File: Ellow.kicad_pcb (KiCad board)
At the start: 2 copper layers, 24.3 x 40.6 mm, 23 parts, among them J1 USB_C_Receptacle_USB2.0, J2 M_2_AKey_KB, Q1 A03407, Q2 A03407, U1 AP2112K-3.3, U2 E73-2G4M08S1C, U3 LN2054Y42AMR, Y1 32.768kHz

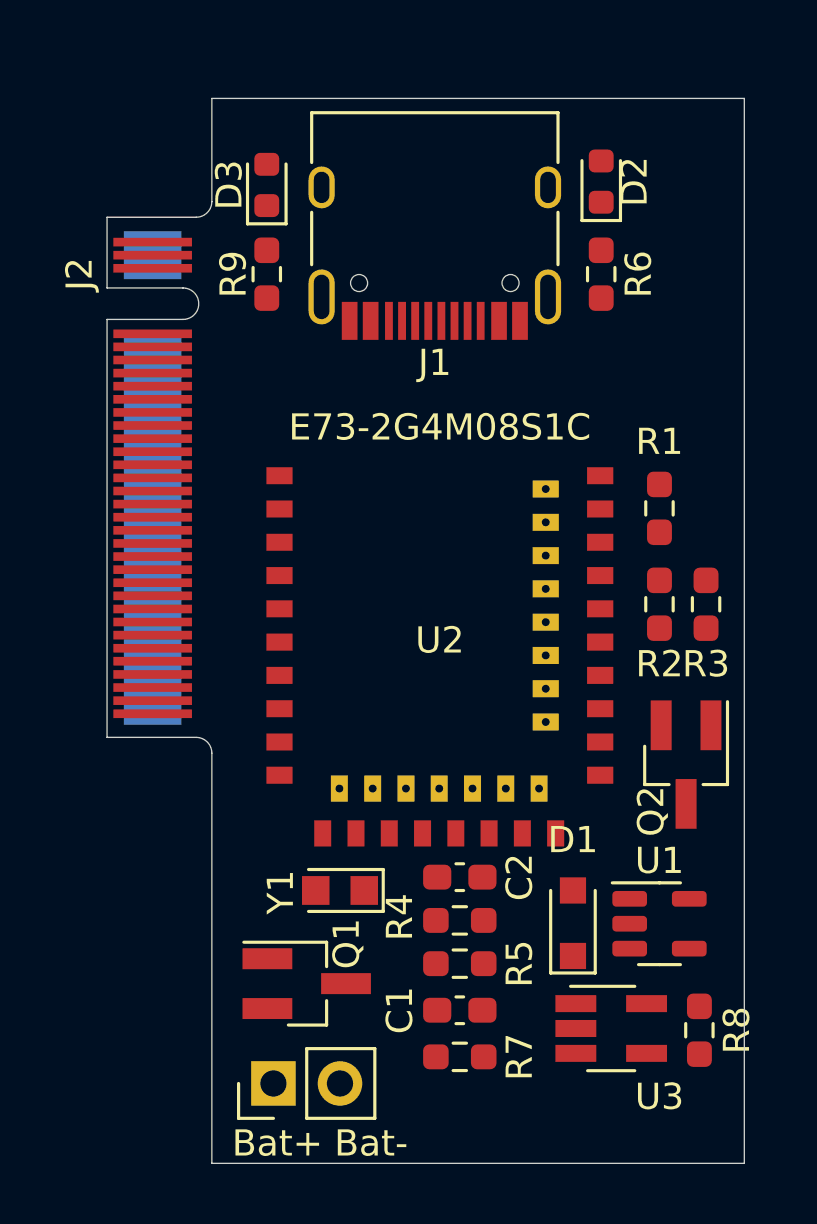
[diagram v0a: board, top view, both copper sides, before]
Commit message: starting to look at routing
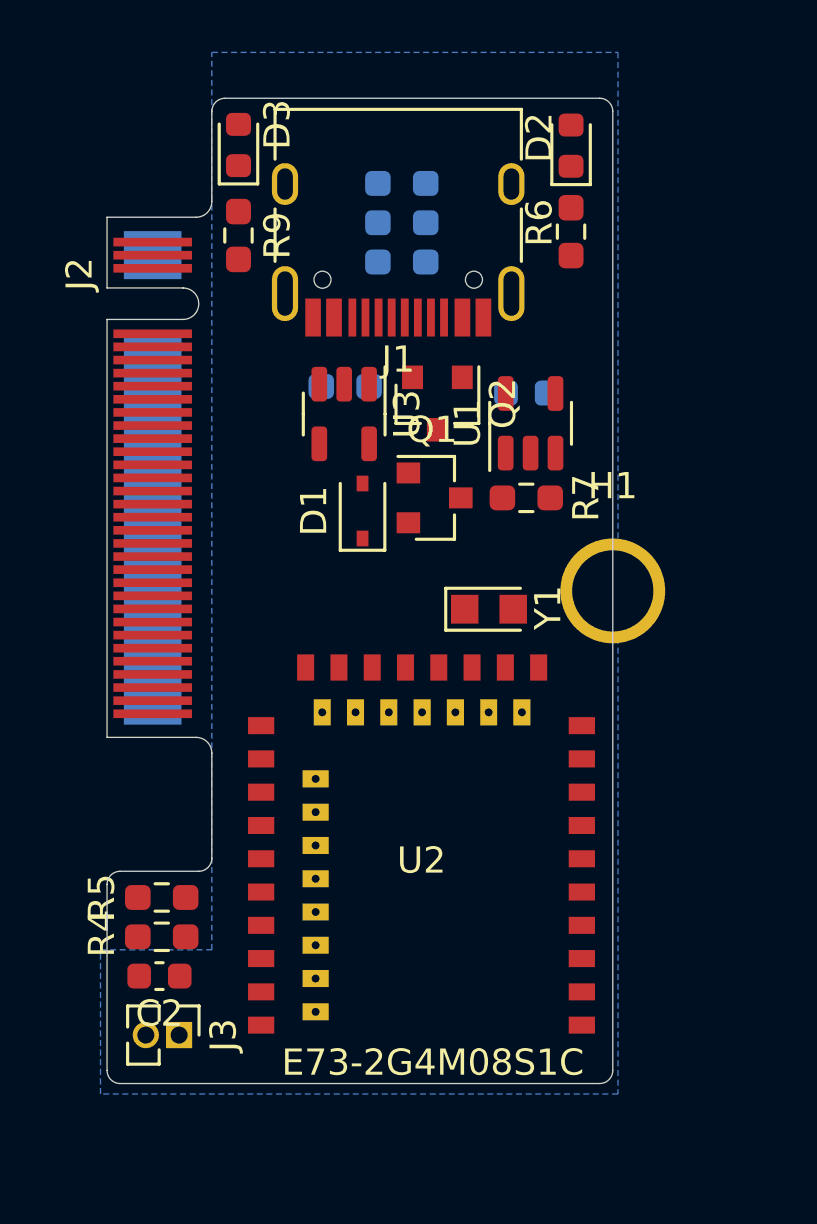
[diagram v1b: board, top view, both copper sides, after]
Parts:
- added H1: MountingHole, ellow:MountingHole_M.2_3mm, F.Cu at (244.1, 107.2)
- C1: footprint Capacitor_SMD:C_0603_1608Metric_Pad1.08x0.95mm_HandSolder -> Capacitor_SMD:C_0603_1608Metric; moved to B.Cu
- C2: footprint Capacitor_SMD:C_0603_1608Metric_Pad1.08x0.95mm_HandSolder -> Capacitor_SMD:C_0603_1608Metric
- D1: footprint Diode_SMD:D_SOD-323_HandSoldering -> Diode_SMD:D_SOD-323
- J3: renamed from Bat+ Bat-; footprint Connector_PinHeader_2.54mm:PinHeader_1x02_P2.54mm_Vertical -> Connector_PinHeader_1.27mm:PinHeader_1x02_P1.27mm_Vertical
- Q1, Q2: footprint Package_TO_SOT_SMD:SOT-23_Handsoldering -> Package_TO_SOT_SMD:SOT-23
- R1, R2, R3, R8: moved to B.Cu
- U3: footprint Package_TO_SOT_SMD:SOT-23-5_HandSoldering -> Package_TO_SOT_SMD:SOT-23-5
- moved R8 28.0 mm to (233.9, 99.4), turned to 180 degrees
- moved U3 25.6 mm to (233.8, 100.5), turned to 270 degrees
- moved C1 23.7 mm to (240.8, 99.7)
- moved R7 21.5 mm to (240.8, 103.7)
- moved R3 19.8 mm to (236.0, 91.7), turned to 0 degrees
- moved U1 19.7 mm to (241.0, 100.8), turned to 90 degrees
- moved Q1 19.2 mm to (237.3, 103.7)
- moved D1 17.7 mm to (234.5, 104.2)
- moved Q2 16.7 mm to (237.4, 100.1)
- moved R2 16.3 mm to (236.0, 94.7), turned to 180 degrees
- moved R1 14.7 mm to (236.0, 93.2), turned to 0 degrees
- moved Y1 12.1 mm to (239.4, 107.9), turned to 0 degrees
- moved C2 12.1 mm to (226.8, 121.9)
- moved R5 11.7 mm to (226.9, 118.9), turned to 180 degrees
- moved R4 11.4 mm to (226.9, 120.4)
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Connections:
- net Net-(U2-Pad12) renamed P0.26
- net Net-(U2-Pad14) renamed P0.06
- net Net-(U2-Pad20) renamed P0.12
- net Net-(U2-Pad22) renamed 90.07
- net Net-(U2-Pad34) renamed P0.22
- net Net-(U2-Pad36) renamed P1.00
- net Net-(U2-Pad38) renamed P1.02
- net Net-(U2-Pad40) renamed P1.04
- J2 pad 1: (no net) -> GND
- J2 pad 16: (no net) -> P0.31
- J2 pad 17: (no net) -> P0.30
- J2 pad 18: (no net) -> Net-(J2-Pad18)
- J2 pad 19: (no net) -> Net-(J2-Pad19)
- J2 pad 2: (no net) -> EXT_VCC
- J2 pad 20: (no net) -> P0.29
- J2 pad 21: (no net) -> P0.02
- J2 pad 22: (no net) -> Net-(J2-Pad22)
- J2 pad 23: (no net) -> Net-(J2-Pad23)
- J2 pad 24: (no net) -> P1.13
- J2 pad 25: (no net) -> GND
- J2 pad 26: (no net) -> Net-(J2-Pad26)
- J2 pad 27: (no net) -> Net-(J2-Pad27)
- J2 pad 28: (no net) -> P0.03
- J2 pad 29: (no net) -> P0.28
- J2 pad 3: (no net) -> Net-(J2-Pad3)
- J2 pad 30: (no net) -> Net-(J2-Pad30)
- J2 pad 31: (no net) -> Net-(J2-Pad31)
- J2 pad 32: (no net) -> P1.11
- J2 pad 33: (no net) -> P1.06
- J2 pad 34: (no net) -> Net-(J2-Pad34)
- J2 pad 35: (no net) -> Net-(J2-Pad35)
- J2 pad 36: (no net) -> P0.10
- J2 pad 37: (no net) -> P0.09
- J2 pad 38: (no net) -> Net-(J2-Pad38)
- J2 pad 39: (no net) -> Net-(J2-Pad39)
- J2 pad 4: (no net) -> Net-(J2-Pad4)
- J2 pad 40: (no net) -> GND
- J2 pad 41: (no net) -> P0.24
- J2 pad 42: (no net) -> Net-(J2-Pad42)
- J2 pad 43: (no net) -> Net-(J2-Pad43)
- J2 pad 44: (no net) -> P0.13
- J2 pad 45: (no net) -> P0.20
- J2 pad 46: (no net) -> Net-(J2-Pad46)
- J2 pad 47: (no net) -> Net-(J2-Pad47)
- J2 pad 48: (no net) -> P0.17
- J2 pad 49: (no net) -> P0.15
- J2 pad 5: (no net) -> VBAT
- J2 pad 50: (no net) -> Net-(J2-Pad50)
- J2 pad 51: (no net) -> Net-(J2-Pad51)
- J2 pad 52: (no net) -> P0.08
- J2 pad 53: (no net) -> GND
- J2 pad 54: (no net) -> Net-(J2-Pad54)
- J2 pad 55: (no net) -> Net-(J2-Pad55)
- J2 pad 56: (no net) -> Net-(J2-Pad56)
- J2 pad 57: (no net) -> Net-(J2-Pad57)
- J2 pad 58: (no net) -> Net-(J2-Pad58)
- J2 pad 59: (no net) -> Net-(J2-Pad59)
- J2 pad 6: (no net) -> RESET
- J2 pad 60: (no net) -> Net-(J2-Pad60)
- J2 pad 61: (no net) -> Net-(J2-Pad61)
- J2 pad 62: (no net) -> Net-(J2-Pad62)
- J2 pad 63: (no net) -> Net-(J2-Pad63)
- J2 pad 64: (no net) -> Net-(J2-Pad64)
- J2 pad 65: (no net) -> Net-(J2-Pad65)
- J2 pad 66: (no net) -> DATA+
- J2 pad 67: (no net) -> DATA-
- J2 pad 68: (no net) -> Net-(J2-Pad68)
- J2 pad 69: (no net) -> Net-(J2-Pad69)
- J2 pad 7: (no net) -> Net-(J2-Pad7)
- J2 pad 70: (no net) -> SWD
- J2 pad 71: (no net) -> GND
- J2 pad 72: (no net) -> Net-(J2-Pad72)
- J2 pad 73: (no net) -> Net-(J2-Pad73)
- J2 pad 74: (no net) -> SWC
- J2 pad 75: (no net) -> VDD_H
- U2 pad 1: Net-(U2-Pad1) -> P1.11
- U2 pad 10: Net-(U2-Pad10) -> P0.30
- U2 pad 16: Net-(U2-Pad16) -> P0.08
- U2 pad 28: Net-(U2-Pad28) -> P0.15
- U2 pad 3: Net-(U2-Pad3) -> P0.03
- U2 pad 30: Net-(U2-Pad30) -> P0.17
- U2 pad 32: Net-(U2-Pad32) -> P0.20
- U2 pad 33: Net-(U2-Pad33) -> P0.13
- U2 pad 35: Net-(U2-Pad35) -> P0.24
- U2 pad 4: Net-(U2-Pad4) -> P0.28
- U2 pad 41: Net-(U2-Pad41) -> P0.09
- U2 pad 42: Net-(U2-Pad42) -> P1.06
- U2 pad 43: Net-(U2-Pad43) -> P0.10
- U2 pad 6: Net-(U2-Pad6) -> P1.13
- U2 pad 7: Net-(U2-Pad7) -> P0.02
- U2 pad 8: Net-(U2-Pad8) -> P0.29
- U2 pad 9: Net-(U2-Pad9) -> P0.31
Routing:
- added copper zone on B.Cu, net GND
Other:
- board size 24.3 x 40.6 mm -> 19.3 x 37.6 mm
